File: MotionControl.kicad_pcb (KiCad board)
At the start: 2 copper layers, 190 x 80 mm, 176 parts, among them J1 Screw_Terminal_01x02, J10 Screw_Terminal_01x02, J11 Screw_Terminal_01x02, J2 Conn_ARM_JTAG_SWD_10, J3 Screw_Terminal_01x04, J5 Screw_Terminal_01x04, J6 Screw_Terminal_01x04, J7 Screw_Terminal_01x04, J8 Screw_Terminal_01x02, J9 Screw_Terminal_01x02, P1 USB_C_Plug_USB2.0, Q1 2N7002, Q10 Q_NMOS_DGS, Q11 Q_NMOS_DGS, Q12 Q_NMOS_DGS, Q13 Q_NMOS_DGS, Q14 Q_NMOS_DGS, Q15 Q_NMOS_DGS, Q16 Q_NMOS_DGS, Q17 Q_NMOS_DGS, Q18 Q_NMOS_DGS, Q19 Q_NMOS_DGS, Q2 Q_NMOS_DGS, Q20 Q_NMOS_DGS, Q21 Q_NMOS_DGS, Q22 Q_NMOS_DGS, Q23 Q_NMOS_DGS, Q24 Q_NMOS_DGS, Q25 Q_NMOS_DGS, Q26 Q_NMOS_DGS, Q27 Q_NMOS_DGS, Q28 Q_NMOS_DGS, Q29 Q_NMOS_DGS, Q3 Q_NMOS_DGS, Q30 Q_NMOS_DGS, Q31 Q_NMOS_DGS, Q32 Q_NMOS_DGS, Q33 Q_NMOS_DGS, Q4 Q_NMOS_DGS, Q5 Q_NMOS_DGS, Q6 Q_NMOS_DGS, Q7 Q_NMOS_DGS, Q8 Q_NMOS_DGS, Q9 Q_NMOS_DGS, SW1 SW_Push, U1 ATSAMD21J18A-A, U2 AP2112K-3.3, U3 TMC5160A-TA, U4 TMC5160A-TA, U5 TMC5160A-TA, U6 TMC5160A-TA, U7 TC4427, Y1 32.768kHz

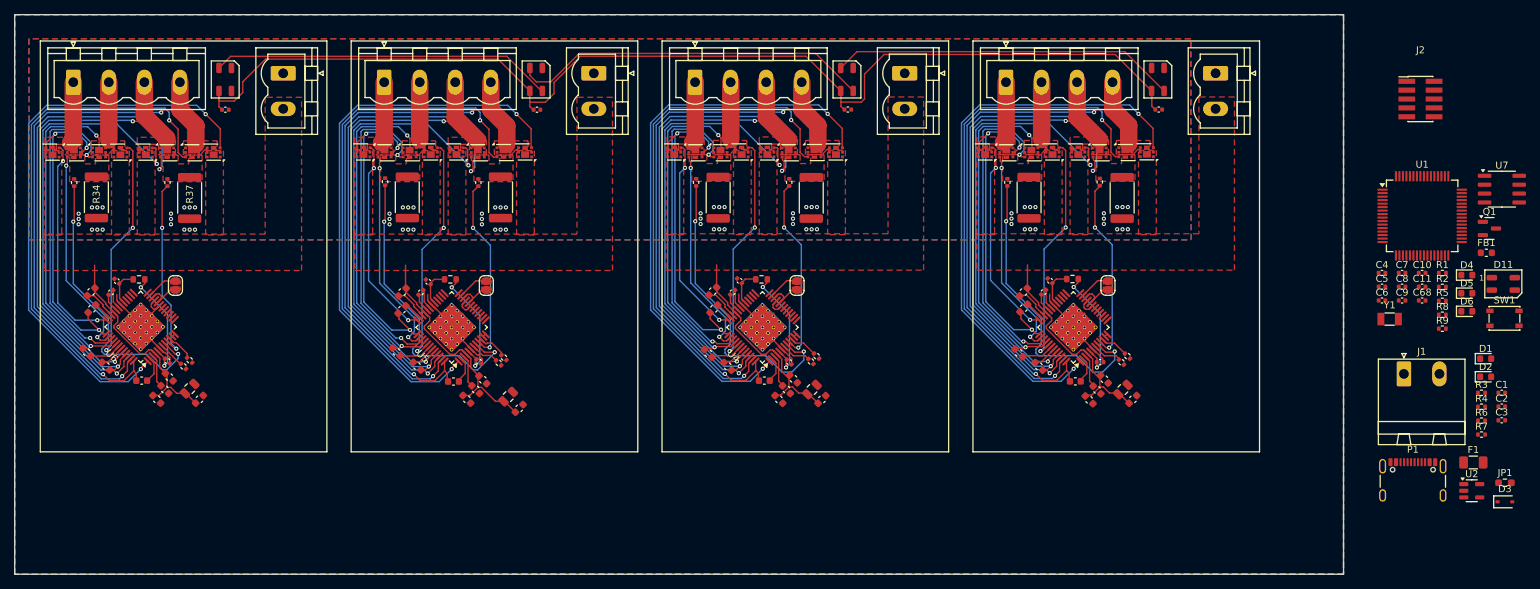
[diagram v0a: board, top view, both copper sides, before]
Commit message: lots of changes for mcu
more routed connections
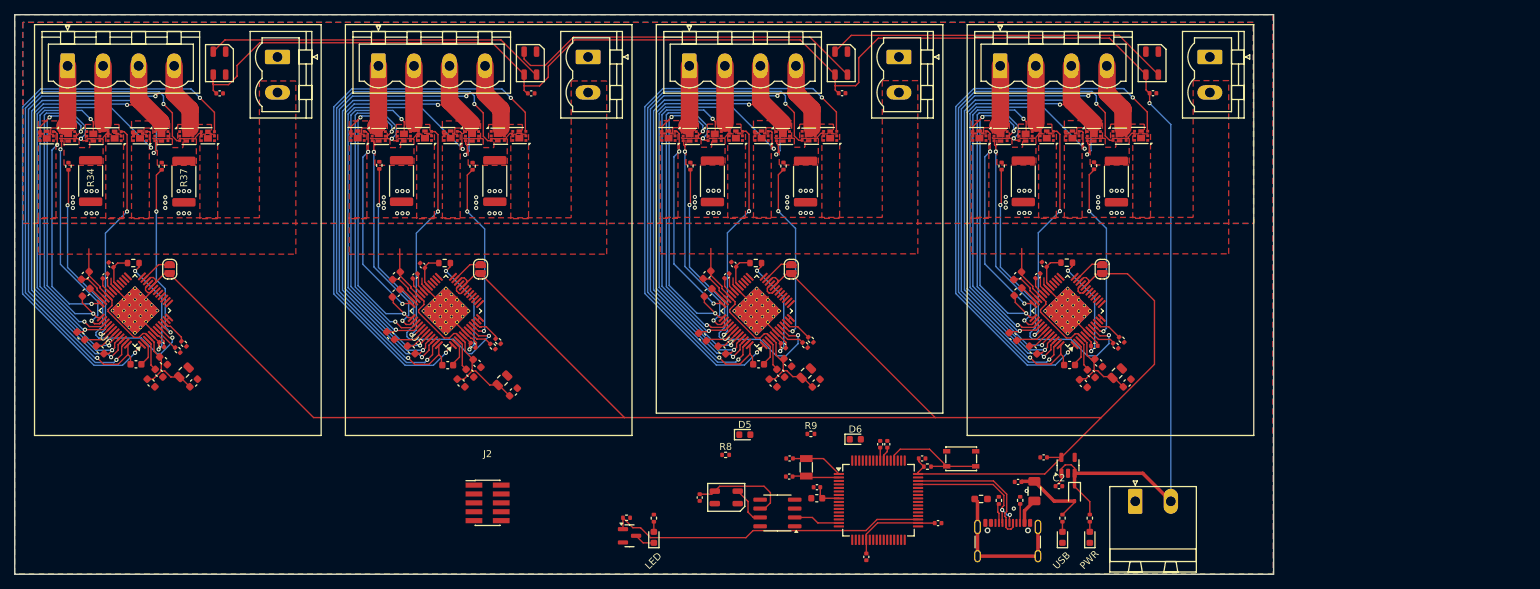
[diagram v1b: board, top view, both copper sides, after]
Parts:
- moved J2 145.3 mm to (100.6, 90.1)
- moved Q1 130.6 mm to (120.9, 94.8)
- moved D4 122.1 mm to (124.4, 95.0), turned to 90 degrees
- moved R5 120.7 mm to (120.5, 92.3), turned to 180 degrees
- moved R2 117.5 mm to (124.4, 92.3), turned to 90 degrees
- moved D11 115.2 mm to (134.8, 89.3)
- moved U7 113.5 mm to (142.1, 91.6), turned to 180 degrees
- moved C68 107.1 mm to (131.0, 89.4), turned to -90 degrees
- moved D5 105.2 mm to (137.4, 80.4)
- moved R8 104.4 mm to (134.7, 83.3)
- moved FB1 102.0 mm to (147.7, 89.5)
- moved R9 91.5 mm to (146.9, 80.3)
- moved D6 89.3 mm to (153.2, 81.0)
- moved C10 89.2 mm to (154.8, 97.8), turned to -90 degrees
- moved C5 89.0 mm to (143.8, 86.4)
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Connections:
- Q1 pad 1: PA17_LED -> PA16_LED
- R5 pad 2: PA17_LED -> PA16_LED
- U1 pad 15: unconnected-(U1-PA06-Pad15) -> PA06_NEOPIX
- U1 pad 35: unconnected-(U1-PA16-Pad35) -> PA16_LED
- U1 pad 36: PA17_LED -> unconnected-(U1-PA17-Pad36)
- U7 pad 2: unconnected-(U7-INA-Pad2) -> PA06_NEOPIX
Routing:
- net +3V3: track 24.4 -> 302.7 mm
- net +5V: track 164.2 -> 266.2 mm, vias 0 -> 1
- net PA16_LED: track 0.00 -> 46.1 mm
- net Net-(JP1-A): track 0.00 -> 21.2 mm
- net /D+: track 0.00 -> 20.2 mm
- net /D-: track 0.00 -> 19.5 mm, vias 0 -> 2
- net /RESETn: track 0.00 -> 16.0 mm
- net VBUS: track 0.00 -> 11.4 mm
- net Net-(U1-PA00): track 0.00 -> 7.49 mm
- net Net-(U1-PA01): track 0.00 -> 6.73 mm
- net PA06_NEOPIX: track 0.00 -> 6.64 mm
- net Net-(D11-DIN): track 0.00 -> 5.66 mm
- net Net-(U1-VDDANA): track 0.00 -> 4.08 mm
- net Net-(F1-Pad1): track 0.00 -> 3.73 mm
- net Net-(D4-K): track 0.00 -> 2.96 mm
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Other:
- board size 190 x 80 mm -> 180 x 80 mm
- board text added: "LED"
- board text added: "PWR"
- board text added: "USB"
